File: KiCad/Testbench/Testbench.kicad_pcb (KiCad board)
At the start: 2 copper layers, 224 x 186 mm, 126 parts, among them J1 Conn_02x03_Counter_Clockwise, J10 Conn_01x02_Pin, J11 Conn_01x02_Pin, J12 Conn_01x02_Pin, J13 Conn_01x02_Pin, J14 Conn_01x02_Pin, J15 Conn_01x02_Pin, J16 Conn_01x02_Pin, J17 Conn_01x02_Pin, J18 Conn_02x03_Counter_Clockwise, J19 Conn_02x02_Top_Bottom, J2 Conn_02x02_Top_Bottom, J20 Conn_02x02_Top_Bottom, J21 Conn_02x02_Top_Bottom, J22 Conn_02x02_Top_Bottom, J23 Conn_02x02_Top_Bottom, J24 Conn_02x02_Top_Bottom, J25 Conn_02x02_Top_Bottom, J26 Conn_02x02_Top_Bottom, J27 Conn_02x02_Top_Bottom, J28 Conn_02x02_Top_Bottom, J29 Conn_02x02_Top_Bottom, J3 Conn_02x02_Top_Bottom, J4 Conn_02x02_Top_Bottom, J6 Conn_02x05_Counter_Clockwise, J7 Conn_01x02_Pin, J8 Conn_01x02_Pin, J9 Conn_02x05_Counter_Clockwise

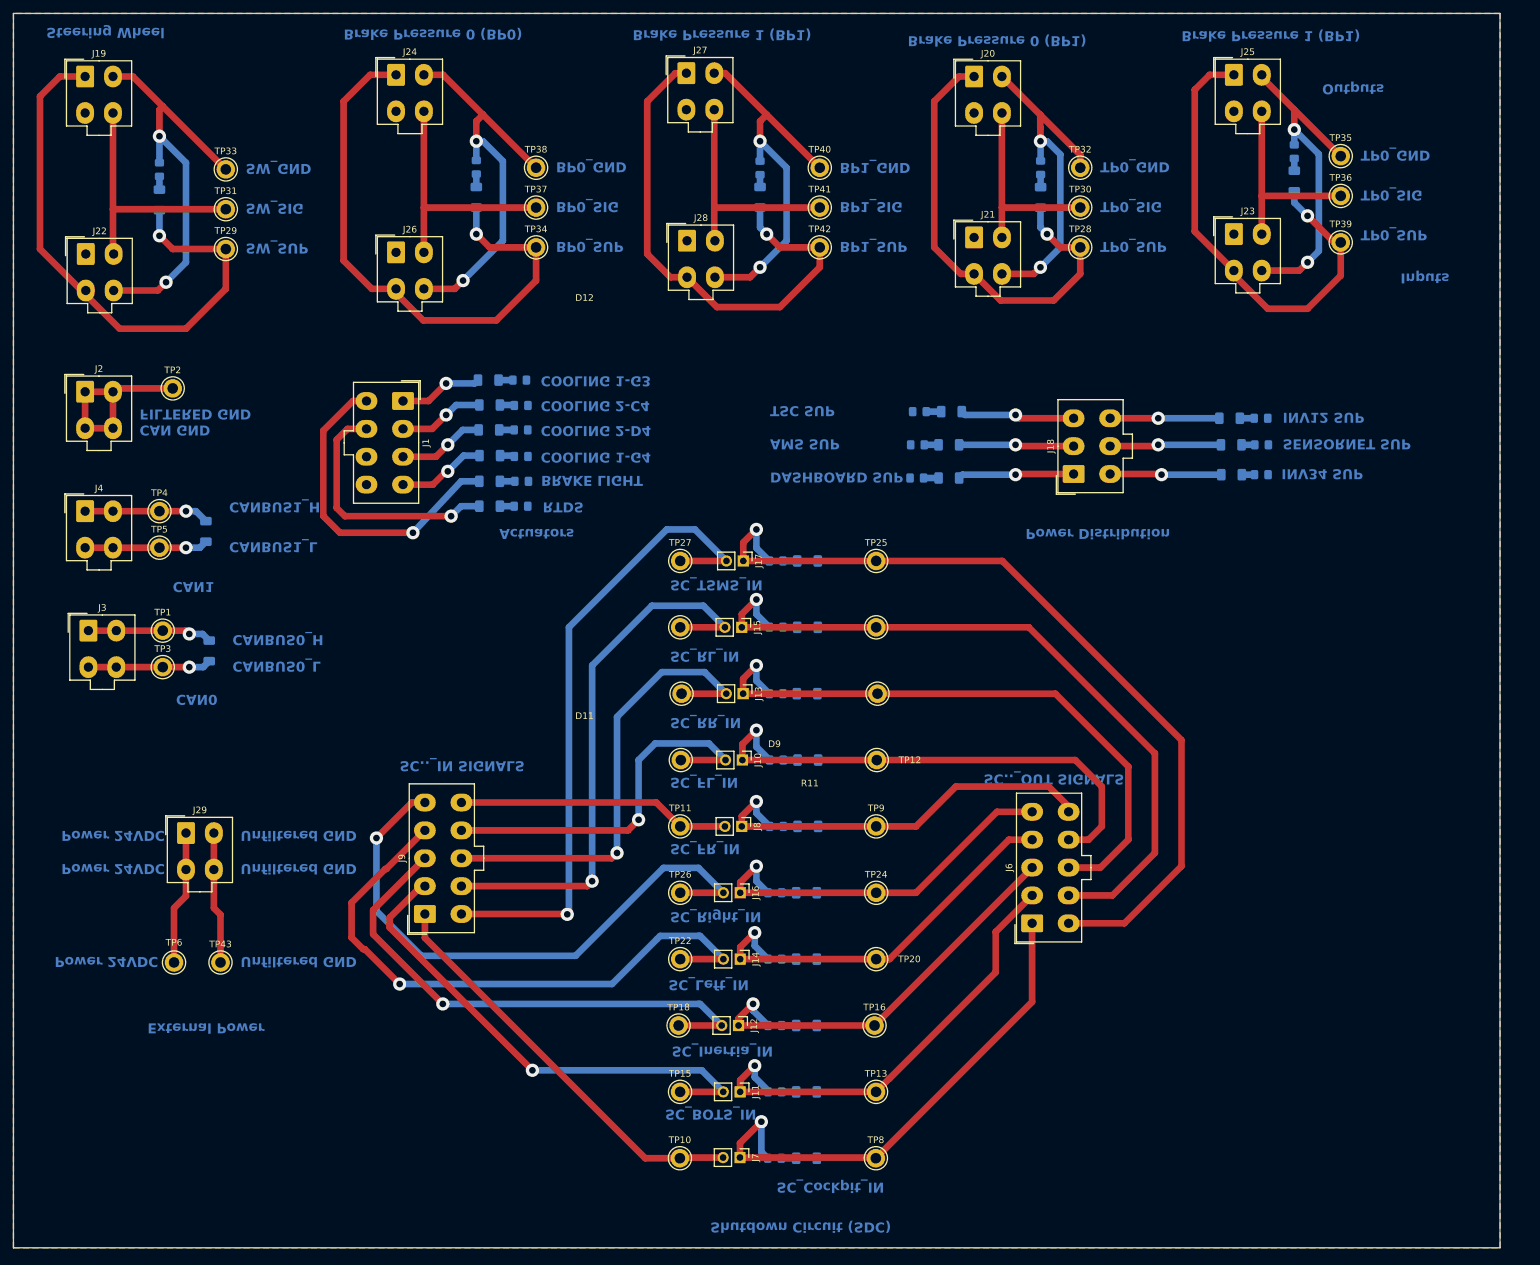
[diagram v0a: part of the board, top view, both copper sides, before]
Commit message: After work 151024
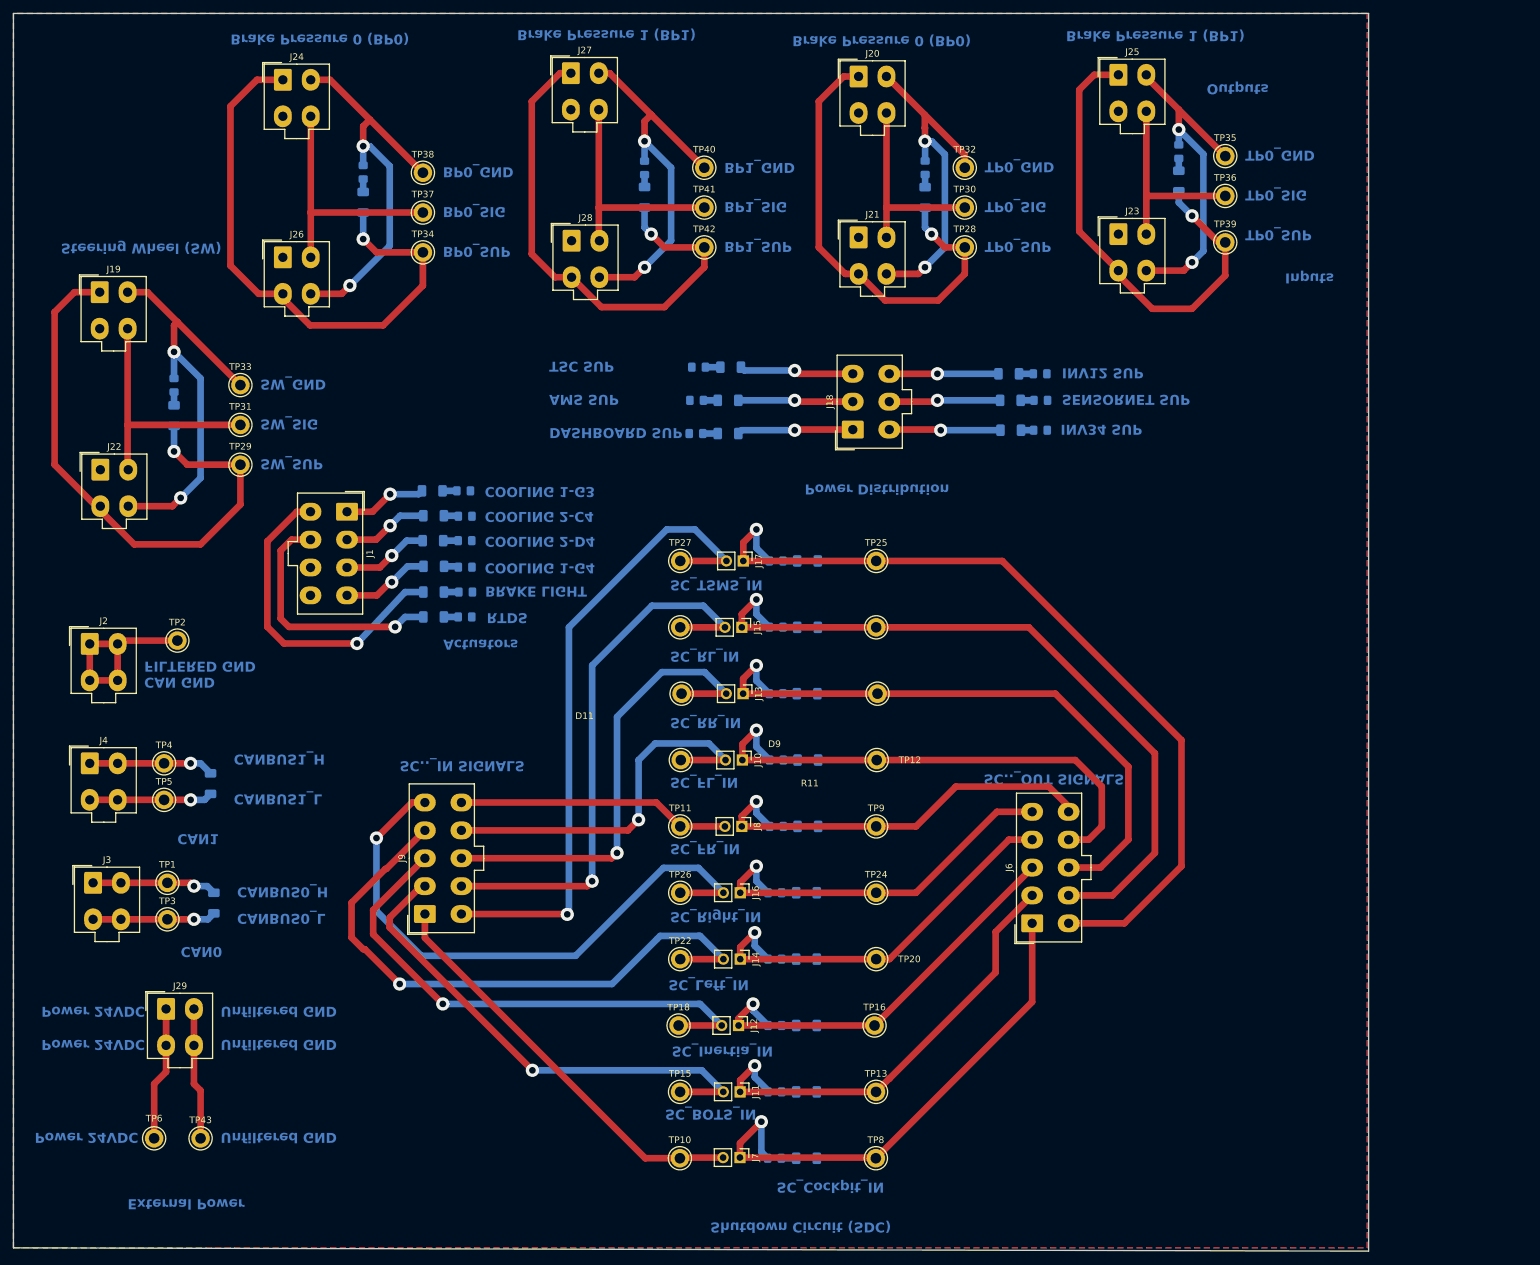
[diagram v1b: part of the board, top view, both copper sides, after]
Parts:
- moved R7 38.0 mm to (42.0, 146.6)
- moved R8 38.0 mm to (41.5, 128.6)
- moved J2 38.0 mm to (23.3, 107.5)
- moved J3 38.0 mm to (23.8, 143.5)
- moved J4 38.0 mm to (23.3, 125.5)
- moved TP1 38.0 mm to (35.0, 143.5)
- moved TP2 38.0 mm to (36.5, 107.0)
- moved TP3 38.0 mm to (35.0, 149.0)
- moved TP4 38.0 mm to (34.5, 125.5)
- moved TP5 38.0 mm to (34.5, 131.0)
- moved D17 33.9 mm to (166.6, 70.8)
- moved D18 33.9 mm to (114.7, 75.8)
- moved D19 33.9 mm to (114.8, 70.8)
- moved D21 33.9 mm to (115.0, 65.8)
- moved D22 33.9 mm to (166.5, 66.8)
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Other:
- board size 224 x 186 mm -> 204.2 x 186.5 mm
- board text added: "Steering Wheel (SW)"
- board text removed: "Brake Pressure 0 (BP1)"
- board text removed: "Steering Wheel"
